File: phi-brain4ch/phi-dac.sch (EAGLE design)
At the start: 156 parts, among them IC1 PCM1792A, IC10 LM317, IC11 LM337, IC2 OPA1632D, IC3 OPA1632D, IC4 OPA1632D, IC6 OPA1632D, IC7 REG1117-5, IC8 ADP3301ARZ-3.3, IC9 MGJ2D121515SC, J1 CUI-RCJ-2123, J5 DC21P, X1 04-JST-B4B-XH-A, X2 04-JST-B4B-XH-A

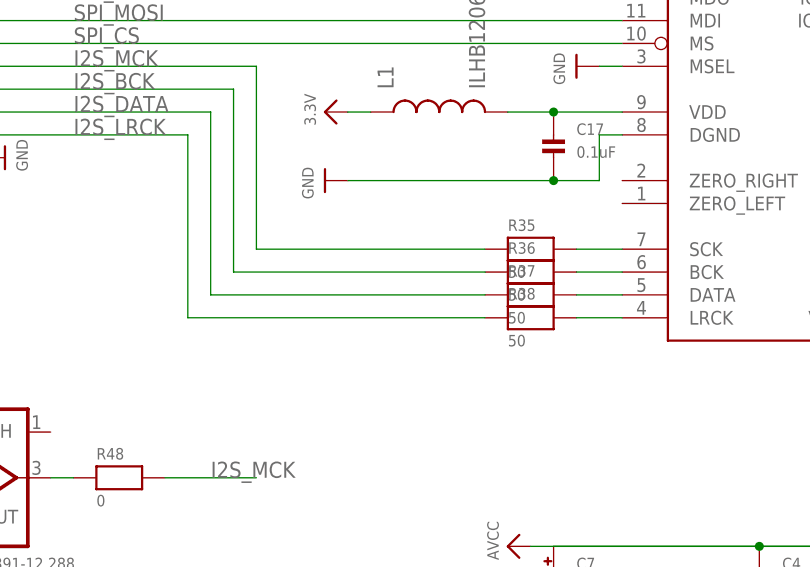
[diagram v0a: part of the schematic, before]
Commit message: wip
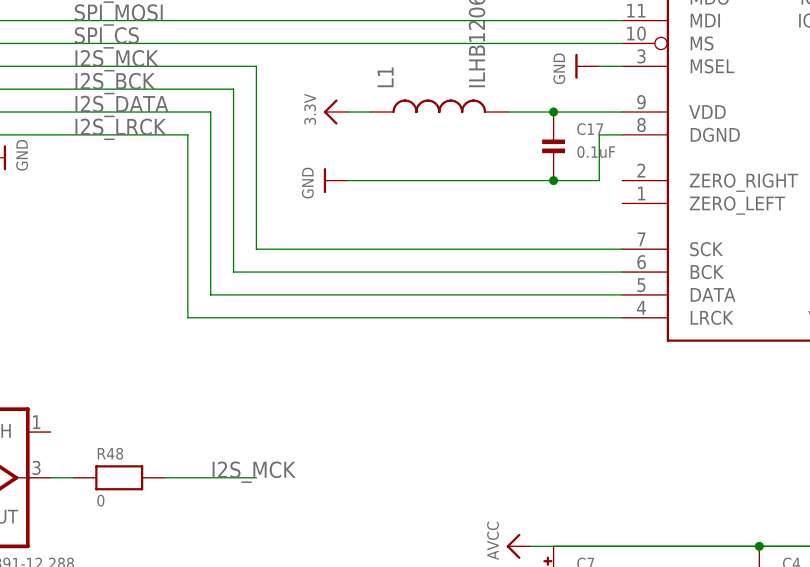
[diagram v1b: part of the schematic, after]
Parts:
- removed R35, R36, R37, R38: 50, microbuilder:RESISTOR_0805
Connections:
- removed net N$43: IC1.BCK, R36.2
- removed net N$44: IC1.DATA, R37.2
- removed net N$45: IC1.LRCK, R38.2
- removed net N$48: IC1.SCK, R35.2
- net I2S_BCK: now also IC1.BCK; no longer R36.1
- net I2S_DATA: now also IC1.DATA; no longer R37.1
- net I2S_LRCK: now also IC1.LRCK; no longer R38.1
- net I2S_MCK: now also IC1.SCK; no longer R35.1
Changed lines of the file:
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@@
 <part name="U$23" library="microbuilder" deviceset="3.3V" device=""/>
 <part name="U$24" library="microbuilder" deviceset="GND" device=""/>
-<part name="R35" library="microbuilder" deviceset="RESISTOR" device="_0805" value="50"/>
-<part name="R36" library="microbuilder" deviceset="RESISTOR" device="_0805" value="50"/>
-<part name="R37" library="microbuilder" deviceset="RESISTOR" device="_0805" value="50"/>
-<part name="R38" library="microbuilder" deviceset="RESISTOR" device="_0805" value="50"/>
 <part name="IC9" library="keves" deviceset="MURATA-MGJ2" device="" value="MGJ2D121515SC"/>
 <part name="U$25" library="microbuilder" deviceset="GND" device=""/>
@@
 <instance part="U$23" gate="G$1" x="40.64" y="142.24" rot="R90"/>
 <instance part="U$24" gate="G$1" x="55.88" y="129.54" rot="R270"/>
-<instance part="R35" gate="G$1" x="50.8" y="109.22"/>
-<instance part="R36" gate="G$1" x="50.8" y="106.68"/>
-<instance part="R37" gate="G$1" x="50.8" y="104.14"/>
-<instance part="R38" gate="G$1" x="50.8" y="101.6"/>
 <instance part="IC9" gate="G$1" x="104.14" y="172.72"/>
 <instance part="U$25" gate="G$1" x="71.12" y="162.56" rot="R270"/>
@@
 </segment>
 </net>
-<net name="N$43" class="0">
-<segment>
-<pinref part="IC1" gate="G$1" pin="BCK"/>
-<pinref part="R36" gate="G$1" pin="2"/>
-<wire x1="55.88" y1="106.68" x2="60.96" y2="106.68" width="0.1524" layer="91"/>
-</segment>
-</net>
-<net name="N$44" class="0">
-<segment>
-<pinref part="IC1" gate="G$1" pin="DATA"/>
-<pinref part="R37" gate="G$1" pin="2"/>
-<wire x1="55.88" y1="104.14" x2="60.96" y2="104.14" width="0.1524" layer="91"/>
-</segment>
-</net>
-<net name="N$45" class="0">
-<segment>
-<pinref part="IC1" gate="G$1" pin="LRCK"/>
-<pinref part="R38" gate="G$1" pin="2"/>
-<wire x1="55.88" y1="101.6" x2="60.96" y2="101.6" width="0.1524" layer="91"/>
-</segment>
-</net>
-<net name="N$48" class="0">
-<segment>
-<pinref part="IC1" gate="G$1" pin="SCK"/>
-<pinref part="R35" gate="G$1" pin="2"/>
-<wire x1="55.88" y1="109.22" x2="60.96" y2="109.22" width="0.1524" layer="91"/>
-</segment>
-</net>
 <net name="I2S_MCK" class="0">
 <segment>
-<pinref part="R35" gate="G$1" pin="1"/>
-<wire x1="45.72" y1="109.22" x2="20.32" y2="109.22" width="0.1524" layer="91"/>
+<wire x1="60.96" y1="109.22" x2="20.32" y2="109.22" width="0.1524" layer="91"/>
 <wire x1="20.32" y1="109.22" x2="20.32" y2="129.54" width="0.1524" layer="91"/>
 <wire x1="20.32" y1="129.54" x2="-10.16" y2="129.54" width="0.1524" layer="91"/>
 <label x="0" y="129.54" size="1.778" layer="95"/>
 <pinref part="SV1" gate="1" pin="9"/>
+<pinref part="IC1" gate="G$1" pin="SCK"/>
 </segment>
 <segment>
@@
 <net name="I2S_BCK" class="0">
 <segment>
-<pinref part="R36" gate="G$1" pin="1"/>
-<wire x1="45.72" y1="106.68" x2="17.78" y2="106.68" width="0.1524" layer="91"/>
+<wire x1="60.96" y1="106.68" x2="17.78" y2="106.68" width="0.1524" layer="91"/>
 <wire x1="17.78" y1="106.68" x2="17.78" y2="127" width="0.1524" layer="91"/>
 <wire x1="17.78" y1="127" x2="-10.16" y2="127" width="0.1524" layer="91"/>
 <label x="0" y="127" size="1.778" layer="95"/>
 <pinref part="SV1" gate="1" pin="7"/>
+<pinref part="IC1" gate="G$1" pin="BCK"/>
 </segment>
 </net>
 <net name="I2S_DATA" class="0">
 <segment>
-<pinref part="R37" gate="G$1" pin="1"/>
-<wire x1="45.72" y1="104.14" x2="15.24" y2="104.14" width="0.1524" layer="91"/>
+<wire x1="60.96" y1="104.14" x2="15.24" y2="104.14" width="0.1524" layer="91"/>
 <wire x1="15.24" y1="104.14" x2="15.24" y2="124.46" width="0.1524" layer="91"/>
 <wire x1="15.24" y1="124.46" x2="-10.16" y2="124.46" width="0.1524" layer="91"/>
 <label x="0" y="124.46" size="1.778" layer="95"/>
 <pinref part="SV1" gate="1" pin="5"/>
+<pinref part="IC1" gate="G$1" pin="DATA"/>
 </segment>
 </net>
 <net name="I2S_LRCK" class="0">
 <segment>
-<pinref part="R38" gate="G$1" pin="1"/>
-<wire x1="45.72" y1="101.6" x2="12.7" y2="101.6" width="0.1524" layer="91"/>
+<wire x1="60.96" y1="101.6" x2="12.7" y2="101.6" width="0.1524" layer="91"/>
 <wire x1="12.7" y1="101.6" x2="12.7" y2="121.92" width="0.1524" layer="91"/>
 <wire x1="12.7" y1="121.92" x2="-10.16" y2="121.92" width="0.1524" layer="91"/>
 <label x="0" y="121.92" size="1.778" layer="95"/>
 <pinref part="SV1" gate="1" pin="3"/>
-</segment>
-</net>
+<pinref part="IC1" gate="G$1" pin="LRCK"/>
+</segment>
+</net>
